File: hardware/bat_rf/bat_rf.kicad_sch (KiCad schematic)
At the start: 87 parts, among them J1 USB_C_Receptacle_PowerOnly_6P, J2 Conn_01x04, Q1 NMOS, Q2 PMOS, Q3 NMOS, SW2 RESET, SW3 SW_MEC_5E, U2 IP2325_5M_WHJC, U3 ESP8684-WROOM-02UC, U4 AMS1117, U5 AMS1117

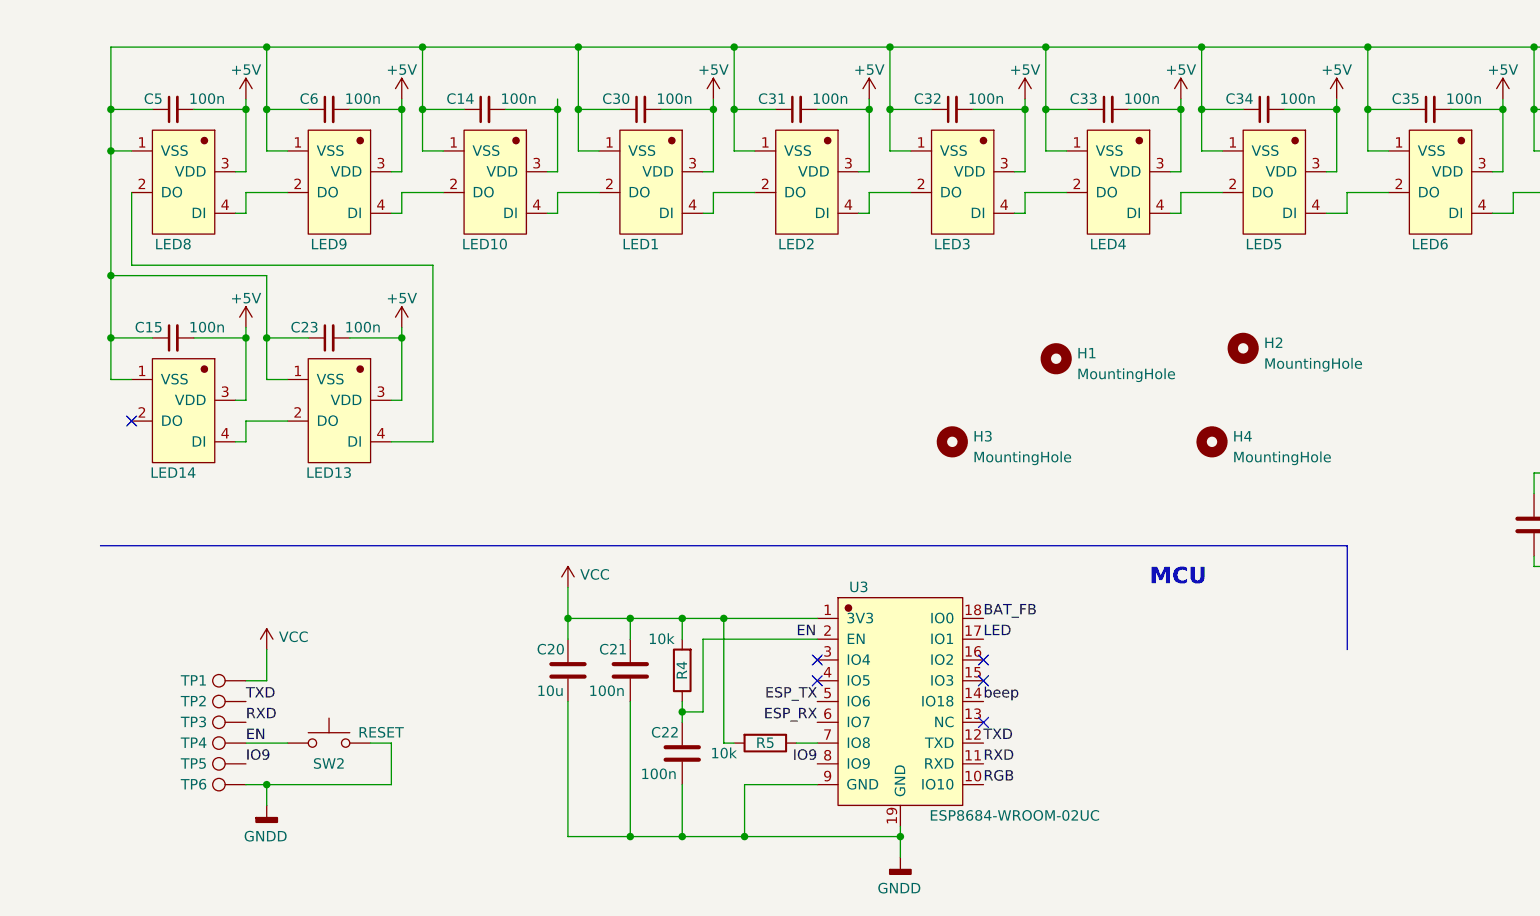
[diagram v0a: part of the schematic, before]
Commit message: update rfBat
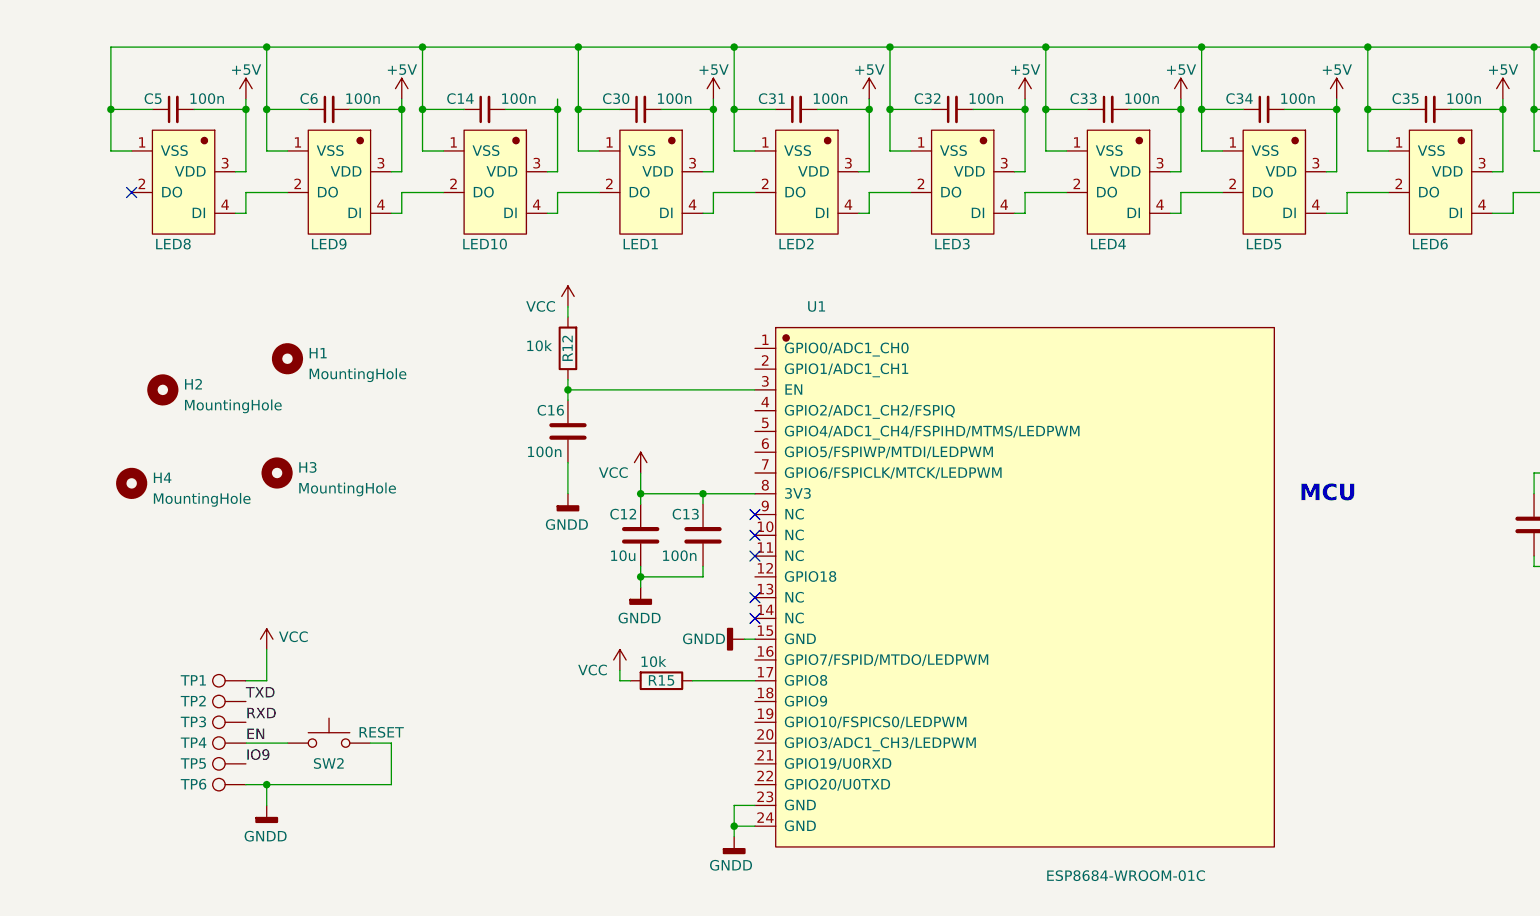
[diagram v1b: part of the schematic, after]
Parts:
- removed C15, C23: 100n, Capacitor_SMD:C_0603_1608Metric_Pad1.08x0.95mm_HandSolder, symbol Device:C_Small
- removed C20: 10u, Capacitor_SMD:C_0805_2012Metric_Pad1.18x1.45mm_HandSolder, symbol Device:C
- removed C21, C22: 100n, Capacitor_SMD:C_0603_1608Metric_Pad1.08x0.95mm_HandSolder, symbol Device:C
- removed LED13, LED14: XL-4020RGBC-WS2812B, bat_rf:LED-SMD_4P-L4.0-W1.7_M4020-03003-RGB-862-001, symbol bat_rf:XL-4020RGBC-WS2812B
- removed R4, R5: 10k, Resistor_SMD:R_0603_1608Metric_Pad0.98x0.95mm_HandSolder, symbol Device:R
- removed U3: ESP8684-WROOM-02UC, bat_rf:WIFIM-SMD_19P-L18.0-W14.3-P1.50_ESP8684-WROOM-02UC, symbol bat_rf:ESP8684-WROOM-02UC
- added C12: 10u, Capacitor_SMD:C_0805_2012Metric_Pad1.18x1.45mm_HandSolder, symbol Device:C
- added C13, C16: 100n, Capacitor_SMD:C_0603_1608Metric_Pad1.08x0.95mm_HandSolder, symbol Device:C
- added R12, R15: 10k, Resistor_SMD:R_0603_1608Metric_Pad0.98x0.95mm_HandSolder, symbol Device:R
- added U1: ESP8684-WROOM-01C, bat_rf:WIRELM-SMD_ESP8684-WROOM0-1C, symbol bat_rf:ESP8684-WROOM-01C
- C1, C3, C8, C9: footprint (none) -> Capacitor_SMD:C_0603_1608Metric_Pad1.08x0.95mm_HandSolder
- C11, C2, C4, C7: footprint (none) -> Capacitor_SMD:C_0805_2012Metric_Pad1.18x1.45mm_HandSolder
- Q2, Q3: footprint (none) -> Package_TO_SOT_SMD:SOT-23
- R11: footprint (none) -> Button_Switch_SMD:SW_SPST_B3S-1000
- R8: footprint (none) -> Resistor_SMD:R_0603_1608Metric_Pad0.98x0.95mm_HandSolder
- SW3: footprint (none) -> Button_Switch_SMD:SW_Push_1P1T_NO_6x6mm_H9.5mm
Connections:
- net GNDD: now also C12.2, C13.2, C16.2, U1.15 (GND), U1.23 (GND), U1.24 (GND)
- net VCC: now also C12.1, C13.1, R12.2, R15.2, U1.8 (3V3)
- new net: C16.1, R12.1, U1.3 (EN)
- new net: R15.1, U1.17 (GPIO8)
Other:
- moved on the sheet: H1, H2, H3, H4
